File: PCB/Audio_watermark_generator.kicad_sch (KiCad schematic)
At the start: 33 parts, among them SW1 SW_Push_DPDT, U1 STM32G431KBTx, U2 TL072, U3 TL072, U4 PAM8303, U5 TL072, U6 TL072, U7 TL072, U8 TL072, U9 TL072

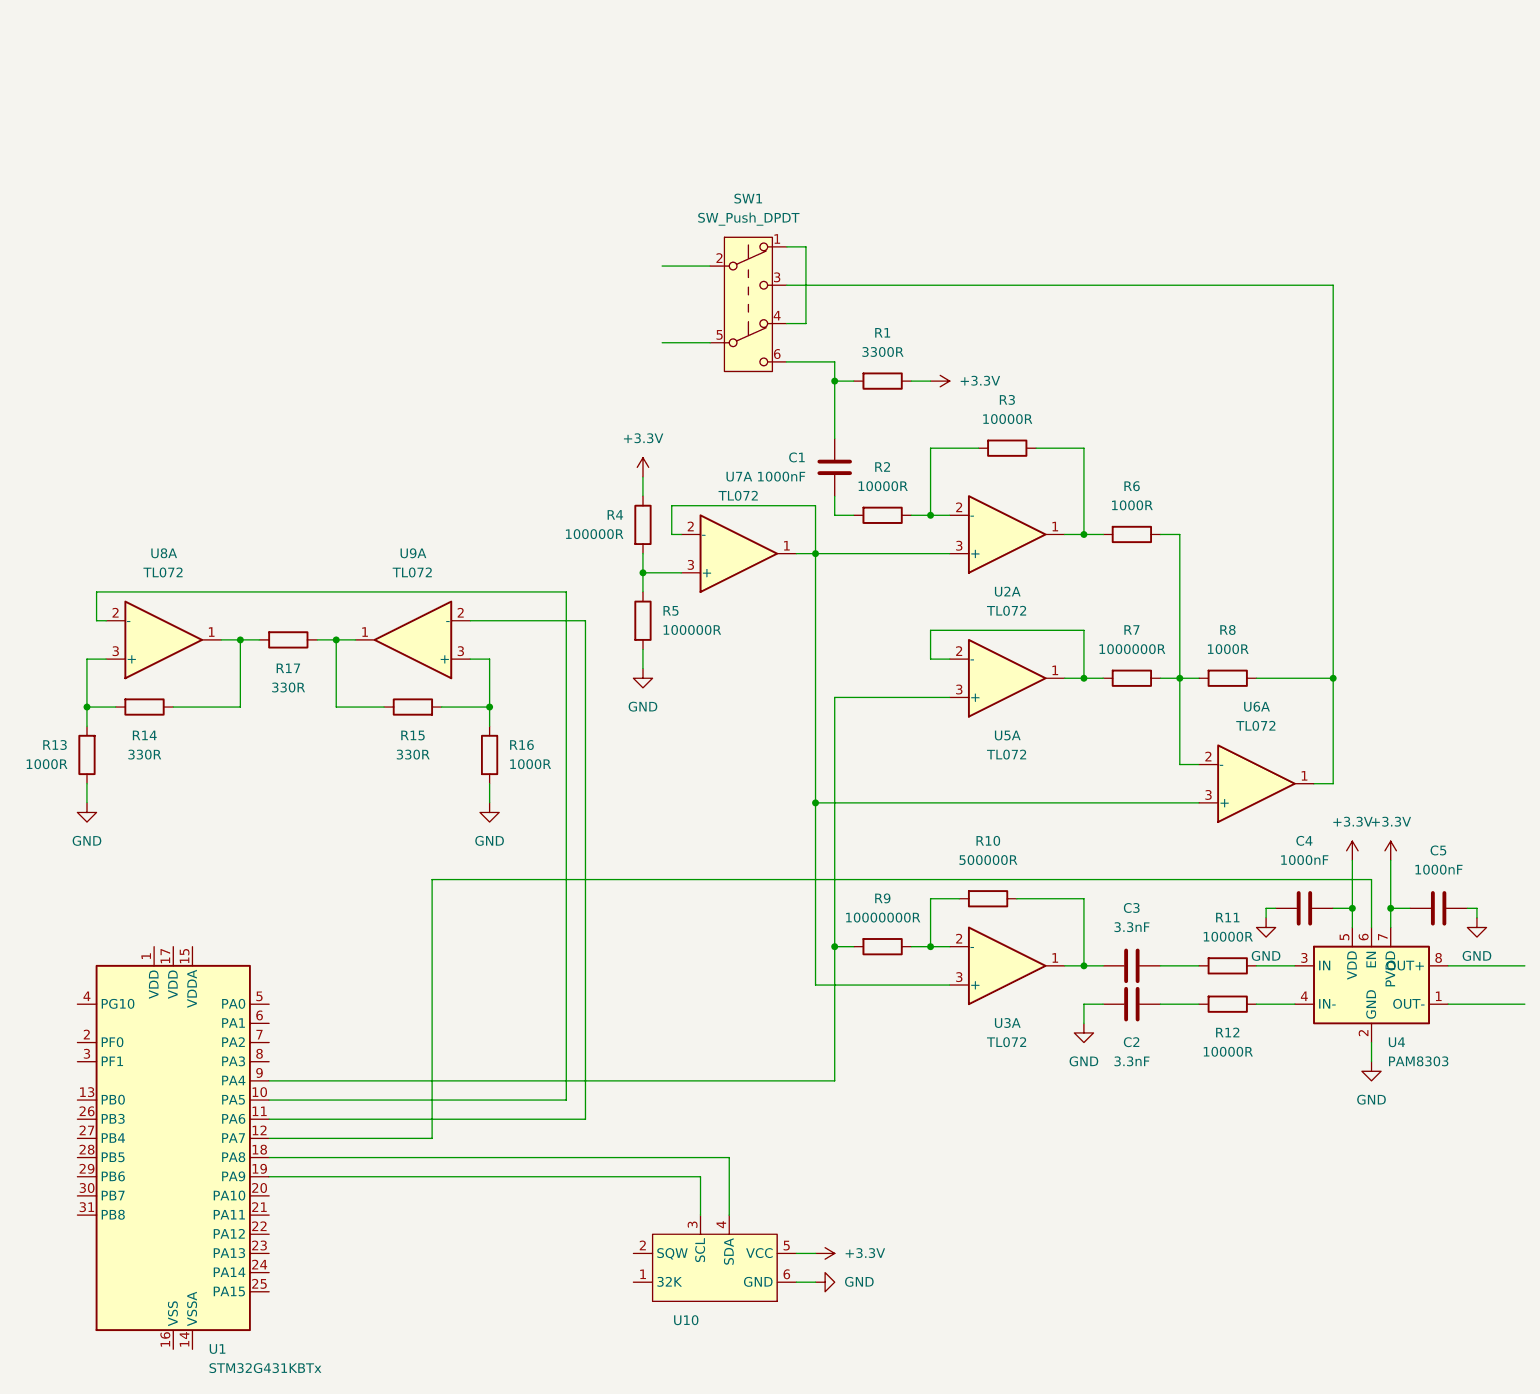
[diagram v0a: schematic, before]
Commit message: Final PCB design with all files included
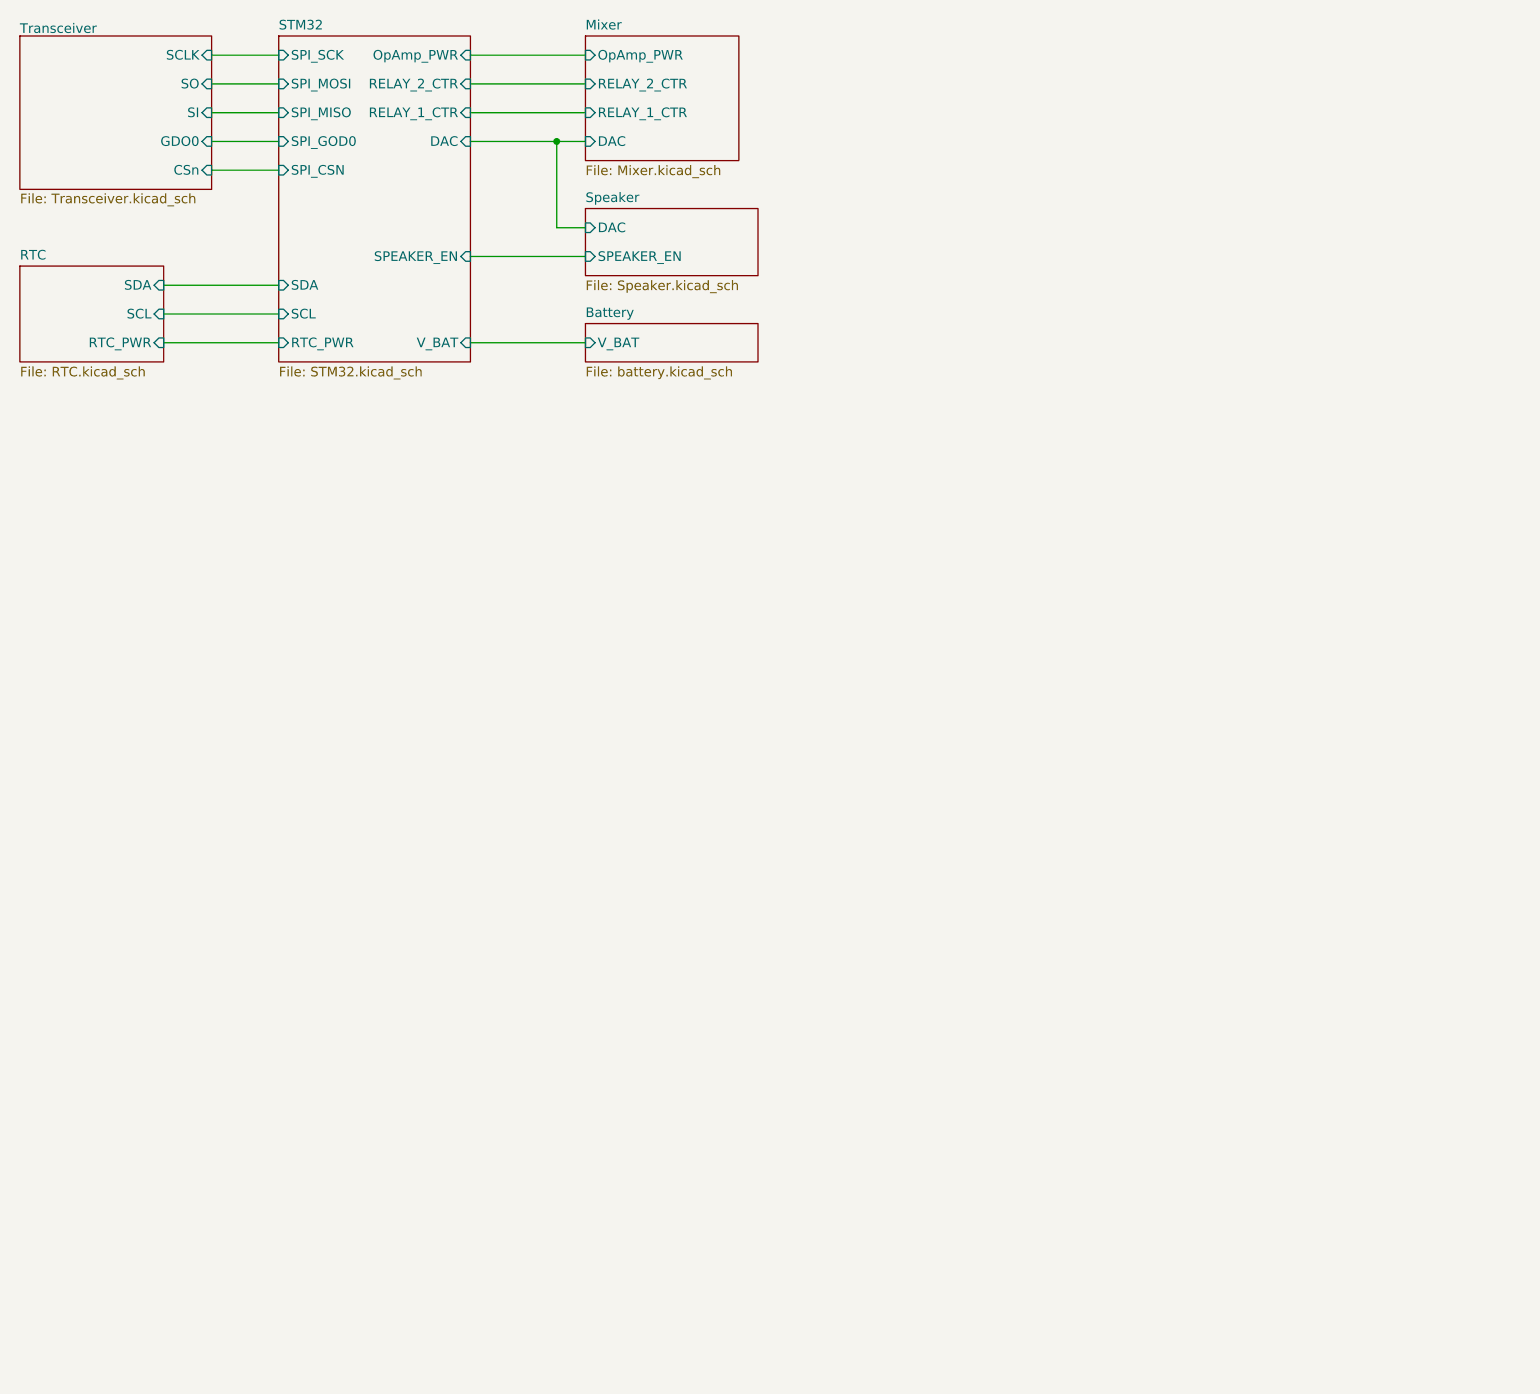
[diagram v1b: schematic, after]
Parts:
- removed C1, C4, C5: 1000nF, Capacitor_SMD:C_0805_2012Metric_Pad1.18x1.45mm_HandSolder, symbol Device:C
- removed C2, C3: 3.3nF, Capacitor_SMD:C_0805_2012Metric_Pad1.18x1.45mm_HandSolder, symbol Device:C
- removed R1: 3300R, Resistor_SMD:R_0805_2012Metric_Pad1.20x1.40mm_HandSolder, symbol Device:R
- removed R10: 500000R, Resistor_SMD:R_0805_2012Metric_Pad1.20x1.40mm_HandSolder, symbol Device:R
- removed R11, R12, R2, R3: 10000R, Resistor_SMD:R_0805_2012Metric_Pad1.20x1.40mm_HandSolder, symbol Device:R
- removed R13, R16, R6, R8: 1000R, Resistor_SMD:R_0805_2012Metric_Pad1.20x1.40mm_HandSolder, symbol Device:R
- removed R14, R15, R17: 330R, Resistor_SMD:R_0805_2012Metric_Pad1.20x1.40mm_HandSolder, symbol Device:R
- removed R4, R5: 100000R, Resistor_SMD:R_0805_2012Metric_Pad1.20x1.40mm_HandSolder, symbol Device:R
- removed R7: 1000000R, Resistor_SMD:R_0805_2012Metric_Pad1.20x1.40mm_HandSolder, symbol Device:R
- removed R9: 10000000R, Resistor_SMD:R_0805_2012Metric_Pad1.20x1.40mm_HandSolder, symbol Device:R
- removed SW1: SW_Push_DPDT, symbol Switch:SW_Push_DPDT
- removed U1: STM32G431KBTx, Package_QFP:LQFP-32_7x7mm_P0.8mm, symbol MCU_ST_STM32G4:STM32G431KBTx
- removed U10: ~, Connector_PinHeader_2.54mm:PinHeader_1x06_P2.54mm_Horizontal, symbol Timer_RTC:DS3231_TH
- removed U2, U3, U5, U6, U7, U8, U9: TL072, symbol Amplifier_Operational:TL072
- removed U4: PAM8303, Package_TO_SOT_SMD:SOT-23-6, symbol Amplifier_Audio:PAM8303
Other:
- added sheet Battery (battery.kicad_sch)
- added sheet Mixer (Mixer.kicad_sch)
- added sheet RTC (RTC.kicad_sch)
- added sheet STM32 (STM32.kicad_sch)
- added sheet Speaker (Speaker.kicad_sch)
- added sheet Transceiver (Transceiver.kicad_sch)
- company: (none) -> NTNU
- title: (none) -> CHIRP-SYNC - Audio Synchronization Module
